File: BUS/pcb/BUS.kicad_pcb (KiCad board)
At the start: 2 copper layers, 30.5 x 17.8 mm, 16 parts, among them J1 Conn_01x03, U1 MAX3483, U2 MAX3051, U3 MCP2515-xSO, Y1 Crystal

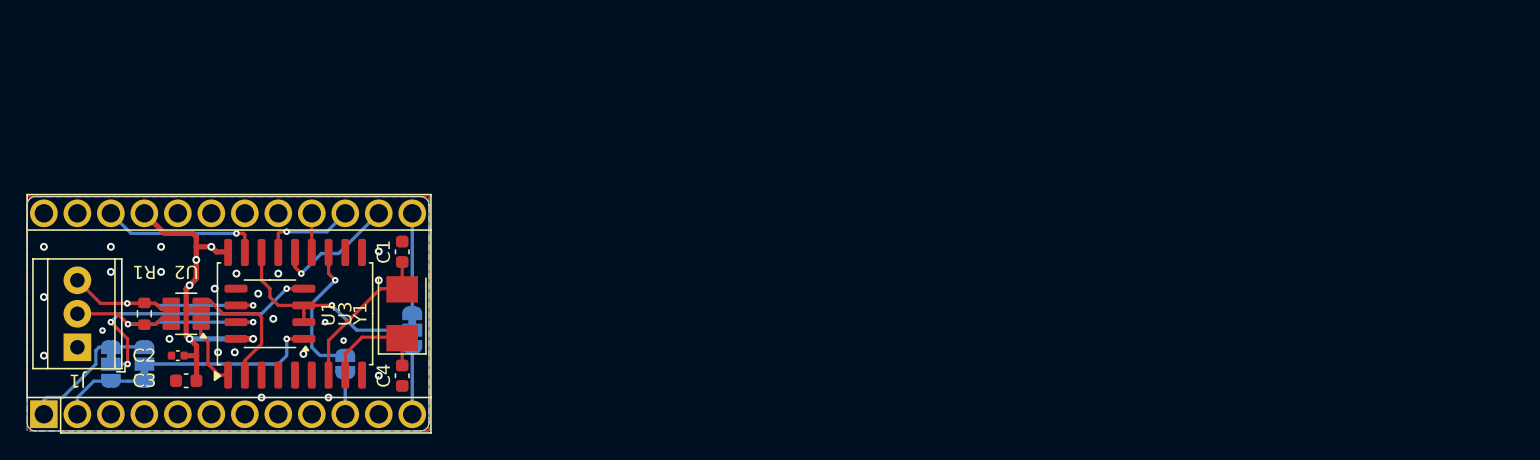
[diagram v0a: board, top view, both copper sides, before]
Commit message: update license
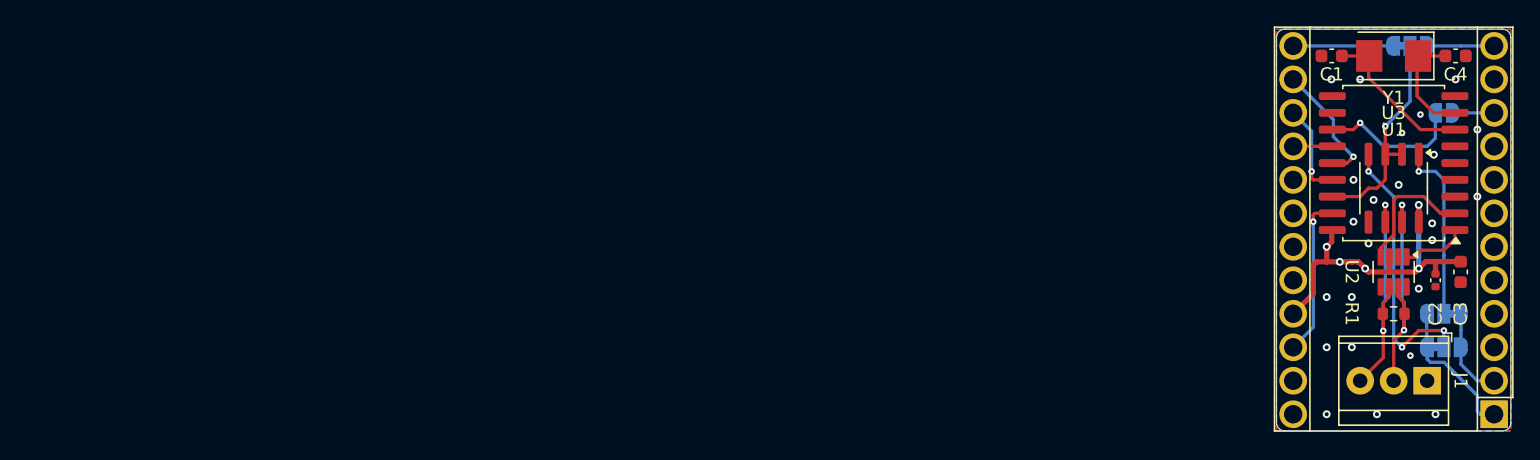
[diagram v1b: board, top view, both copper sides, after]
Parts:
- moved A1 110.0 mm to (216.7, 104.1), turned to 180 degrees
- moved J1 102.4 mm to (211.6, 101.6), turned to 180 degrees
- moved JP2 101.1 mm to (212.9, 99.1), turned to 0 degrees
- moved JP1 98.6 mm to (212.9, 96.5), turned to 180 degrees
- moved C3 97.0 mm to (214.1, 93.3), turned to -90 degrees
- moved C2 95.6 mm to (212.2, 94.0), turned to -90 degrees
- moved R1 94.8 mm to (209.1, 96.5), turned to 180 degrees
- moved U2 91.6 mm to (209.1, 93.3), turned to -90 degrees
- moved U1 85.8 mm to (209.1, 87.0), turned to -90 degrees
- moved JP4 85.5 mm to (212.9, 81.3), turned to 0 degrees
- moved U3 84.1 mm to (209.1, 85.1), turned to 180 degrees
- moved C4 83.5 mm to (213.8, 77.0), turned to 0 degrees
- moved LOGO1 79.7 mm to (208.4, 80.6), turned to -90 degrees
- moved JP3 78.7 mm to (210.3, 76.2), turned to 0 degrees
- moved Y1 77.7 mm to (209.1, 77.0), turned to 180 degrees
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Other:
- board size 30.5 x 17.8 mm -> 17.8 x 30.5 mm
- board text added: "0"
- board text added: "0 mm"
- board text added: "0,01 mm"
- board text added: "0,02"
- board text added: "0,035 mm"
- board text added: "0,1000 mm / 0,0000 mm"
- board text added: "0,2000 mm"
- board text added: "0,71 mm"
- board text added: "0,8000 mm"
- board text added: "1"
- board text added: "17,7800 mm x 30,4800 mm"
- board text added: "2"
- board text added: "3,3"
- board text added: "4,5"
- board text added: "B.Cu"
- board text added: "B.Mask"
- board text added: "B.Paste"
- board text added: "B.Silkscreen"
- board text added: "BOARD CHARACTERISTICS"
- board text added: "Board Thickness:"
- board text added: "Board overall dimensions:"
- board text added: "Bottom Silk Screen"
- board text added: "Bottom Solder Mask"
- board text added: "Bottom Solder Paste"
- board text added: "Castellated pads:"
- board text added: "Color"
- board text added: "Copper Finish:"
- board text added: "Copper Layer Count:"
- board text added: "Dielectric"
- board text added: "Edge card connectors:"
- board text added: "Epsilon R"
- board text added: "F.Cu"
- board text added: "F.Mask"
- board text added: "F.Paste"
- board text added: "F.Silkscreen"
- board text added: "FR4"
- board text added: "Impedance Control:"
- board text added: "Layer Name"
- board text added: "Loss Tangent"
- board text added: "Material"
- board text added: "Min hole diameter:"
- board text added: "Min track/spacing:"
- board text added: "No"
- board text added: "None"
- board text added: "Not specified"
- board text added: "Plated Board Edge:"
- board text added: "Thickness (mm)"
- board text added: "Top Silk Screen"
- board text added: "Top Solder Mask"
- board text added: "Top Solder Paste"
- board text added: "Type"
- board text added: "copper"
- board text added: "core"
